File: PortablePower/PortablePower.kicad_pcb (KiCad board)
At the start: 2 copper layers, 44 x 53 mm, 43 parts, among them IC1 SW6208, J1 USB1130-15-A, J2 2137160001, Q1 CSD17313Q2, Q2 CSD17313Q2, Q3 CSD16406Q3, Q4 CSD16406Q3, U1 USBLC6-2SC6, U2 USBLC6-2SC6, U3 BQ297xy

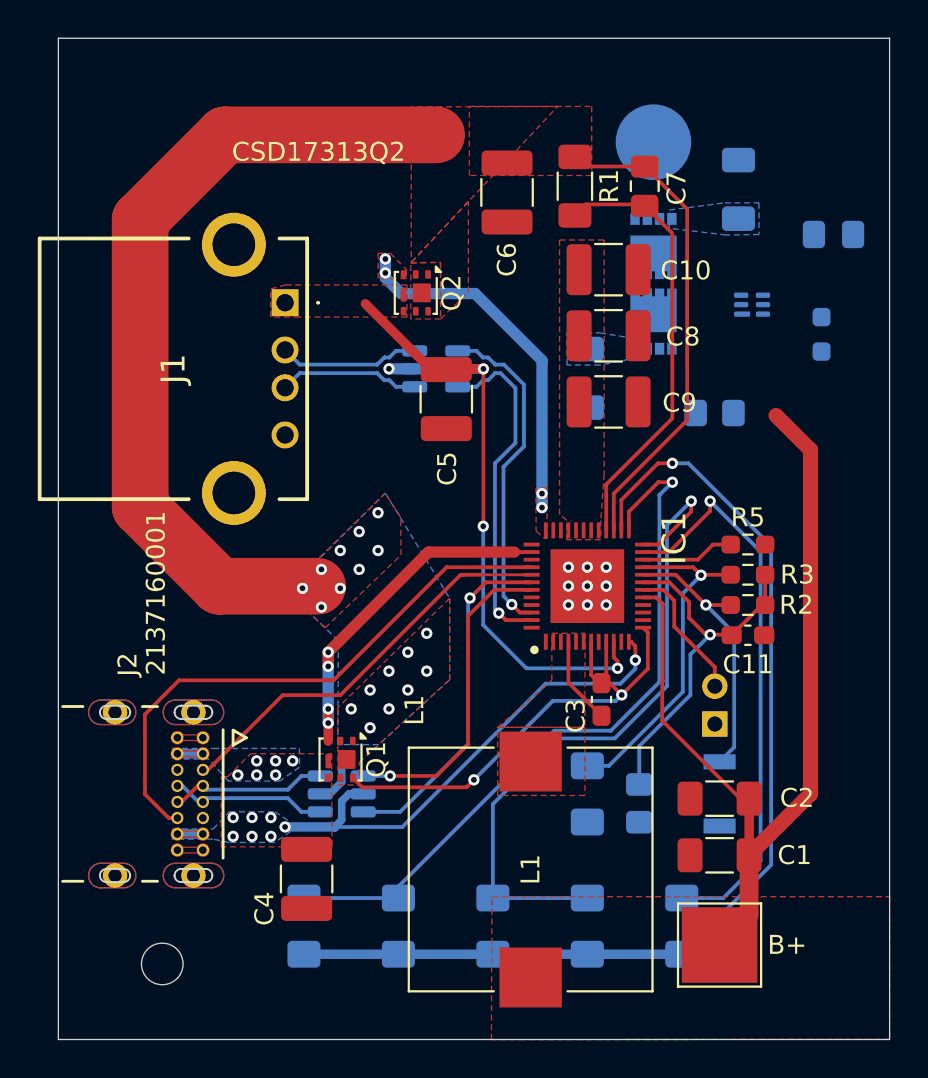
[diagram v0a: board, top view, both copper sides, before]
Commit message: added logo
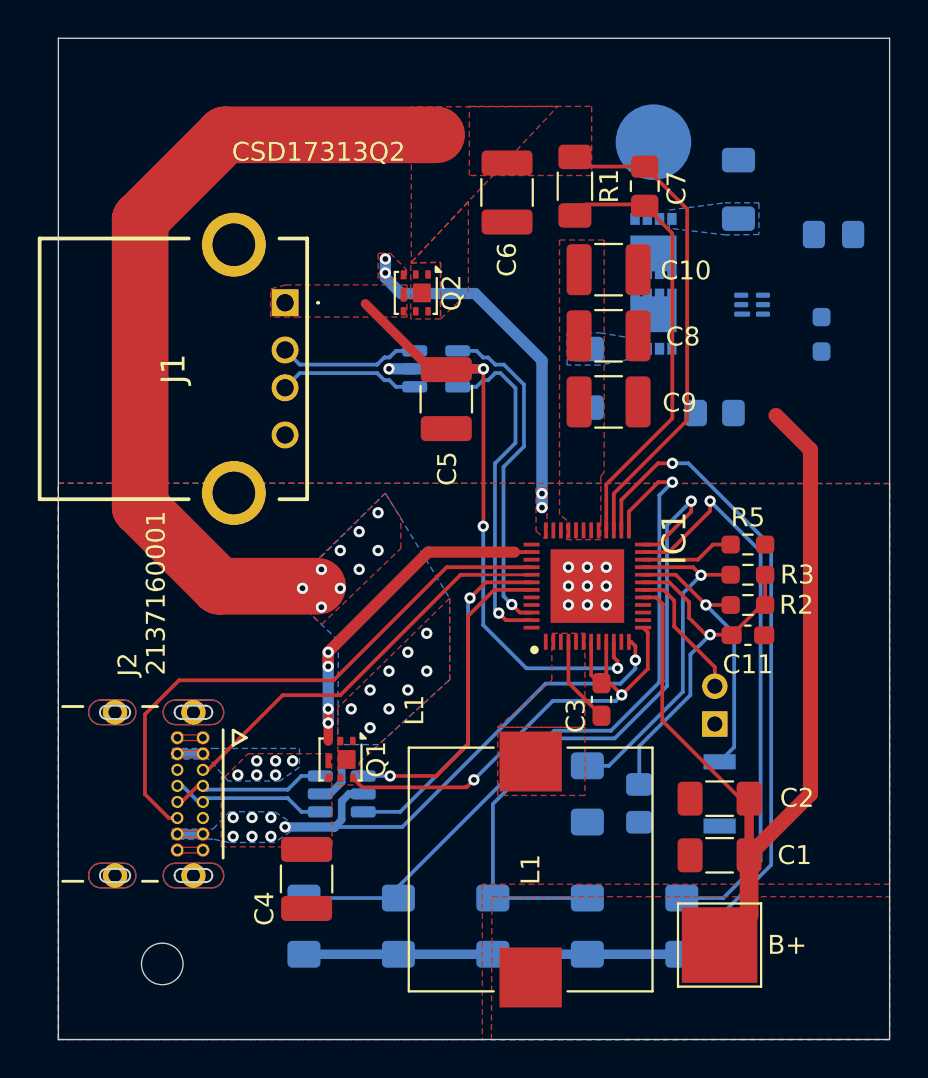
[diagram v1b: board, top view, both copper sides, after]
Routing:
- added copper zone on B.Cu, net GND
- added copper zone on F.Cu, net GND
- added copper zone on B.Cu, net Net-(Q3-G)
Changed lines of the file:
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@@
+	)
+	(segment
+		(start 129.2847 113.5)
+		(end 129.2847 113.4885)
+		(width 0.6)
+		(layer "F.Cu")
+		(net 20)
 	)
 	(segment
@@
 	)
 	(segment
-		(start 129.2847 113.5)
-		(end 134.5847 108.2)
+		(start 129.2847 113.4885)
+		(end 134.5732 108.2)
+		(width 0.6)
+		(layer "F.Cu")
+		(net 20)
+	)
+	(segment
+		(start 134.5732 108.2)
+		(end 139.1412 108.2)
 		(width 0.6)
 		(layer "F.Cu")
@@
 		(end 129.2847 116.5)
 		(width 0.5)
-		(layer "F.Cu")
-		(net 20)
-	)
-	(segment
-		(start 134.5847 108.2)
-		(end 139.1412 108.2)
-		(width 0.6)
 		(layer "F.Cu")
 		(net 20)
@@
 		(name "1")
 		(hatch edge 0.5)
+		(priority 1)
 		(connect_pads yes
 			(clearance 0)
@@
 		(polygon
 			(pts
-				(xy 123.6218 120.101354) (xy 123.952 120.0912) (xy 125.1712 118.872) (xy 129.4638 118.872) (xy 129.489464 123.7996)
-				(xy 123.6218 123.7996)
+				(xy 123.6218 120.101354) (xy 123.820971 120.095229) (xy 125.0442 118.872) (xy 129.4638 118.872)
+				(xy 129.489464 123.7996) (xy 123.6218 123.7996)
 			)
 		)
@@
 		(min_thickness 0.25)
 		(filled_areas_thickness no)
-		(fill
+		(fill yes
 			(thermal_gap 0.5)
 			(thermal_bridge_width 0.5)
@@
 		(name "1")
 		(hatch edge 0.5)
+		(priority 1)
 		(connect_pads yes
 			(clearance 0)
@@
 			(pts
 				(xy 141.9098 107.5436) (xy 141.9098 106.5022) (xy 141.52873 106.218067) (xy 141.52873 91.679346)
-				(xy 143.890941 91.679346) (xy 143.891002 104.0638) (xy 143.7132 106.5276) (xy 143.7132 107.5436)
+				(xy 143.890941 91.679346) (xy 143.891002 103.9876) (xy 143.7132 104.1908) (xy 143.7132 106.5276)
+				(xy 143.7132 107.5436)
 			)
 		)
@@
 	)
 	(zone
+		(net 2)
+		(net_name "GND")
+		(layer "F.Cu")
+		(name "24")
+		(hatch edge 0.5)
+		(connect_pads yes
+			(clearance 0)
+		)
+		(min_thickness 0.25)
+		(filled_areas_thickness no)
+		(fill yes
+			(thermal_gap 0.5)
+			(thermal_bridge_width 0.5)
+			(island_removal_mode 2)
+			(island_area_min 10)
+		)
+		(polygon
+			(pts
+				(xy 114.9858 104.5464) (xy 159.004 104.5718) (xy 159.004 125.7808) (xy 137.4394 125.7808) (xy 137.4394 134.0104)
+				(xy 115.0112 134.0104)
+			)
+		)
+	)
+	(zone
 		(net 22)
 		(net_name "/PD_Control/GATEA1")
@@
 		(polygon
 			(pts
-				(xy 128.1684 111.3028) (xy 129.117893 112.211299) (xy 133.13505 108.3564) (xy 133.1214 106.3752)
+				(xy 128.1684 111.3028) (xy 128.930717 112.032205) (xy 133.132595 108.000046) (xy 133.1214 106.3752)
 				(xy 132.3086 105.0798) (xy 127.21685 110.049492)
 			)
@@
 	)
 	(zone
+		(net 2)
+		(net_name "GND")
+		(layer "B.Cu")
+		(name "1")
+		(hatch edge 0.5)
+		(connect_pads yes
+			(clearance 0)
+		)
+		(min_thickness 0.25)
+		(filled_areas_thickness no)
+		(fill yes
+			(thermal_gap 0.5)
+			(thermal_bridge_width 0.5)
+			(island_removal_mode 2)
+			(island_area_min 10)
+		)
+		(polygon
+			(pts
+				(xy 159.004 104.5718) (xy 159.004 134.0104) (xy 114.9858 134.0104) (xy 114.9858 104.5464)
+			)
+		)
+	)
+	(zone
+		(net 42)
+		(net_name "Net-(Q3-G)")
+		(layer "B.Cu")
+		(name "45")
+		(hatch edge 0.5)
+		(connect_pads yes
+			(clearance 0)
+		)
+		(min_thickness 0.25)
+		(filled_areas_thickness no)
+		(fill yes
+			(thermal_gap 0.5)
+			(thermal_bridge_width 0.5)
+		)
+		(polygon
+			(pts
+				(xy 145.706784 96.929083) (xy 145.706784 97.894283) (xy 143.6784 98.298) (xy 141.9258 98.298) (xy 141.922184 96.598883)
+				(xy 143.6784 96.5962)
+			)
+		)
+	)
+	(zone
+		(net 5)
+		(net_name "/PD_Control/VBUSC")
+		(layer "B.Cu")
+		(name "1")
+		(hatch edge 0.5)
+		(priority 2)
+		(connect_pads yes
+			(clearance 0)
+		)
+		(min_thickness 0.025)
+		(filled_areas_thickness no)
+		(fill yes
+			(thermal_gap 0.5)
+			(thermal_bridge_width 0.5)
+		)
+		(polygon
+			(pts
+				(xy 121.031 119.1514) (xy 121.031 118.5926) (xy 123.19 118.5926) (xy 127.762 118.5926) (xy 127.762 119.5832)
+				(xy 126.7206 120.3198) (xy 123.987338 120.3198) (xy 122.971338 119.1514)
+			)
+		)
+	)
+	(zone
 		(net 43)
 		(net_name "Net-(Q4-G)")
@@
 		(min_thickness 0.25)
 		(filled_areas_thickness no)
-		(fill
-			(thermal_gap 0.5)
-			(thermal_bridge_width 0.5)
-		)
-		(polygon
-			(pts
-				(xy 145.706784 96.929083) (xy 145.706784 97.894283) (xy 143.6784 98.298) (xy 141.9258 98.298) (xy 141.922184 96.598883)
-				(xy 143.6784 96.5962)
-			)
-		)
-	)
-	(zone
-		(net 5)
-		(net_name "/PD_Control/VBUSC")
-		(layer "B.Cu")
-		(name "1")
-		(hatch edge 0.5)
-		(priority 2)
-		(connect_pads yes
-			(clearance 0)
-		)
-		(min_thickness 0.025)
-		(filled_areas_thickness no)
-		(fill yes
-			(thermal_gap 0.5)
-			(thermal_bridge_width 0.5)
-		)
-		(polygon
-			(pts
-				(xy 121.031 119.1514) (xy 121.031 118.5926) (xy 123.19 118.5926) (xy 127.762 118.5926) (xy 127.762 119.5832)
-				(xy 126.7206 120.3198) (xy 123.987338 120.3198) (xy 122.971338 119.1514)
-			)
-		)
-	)
-	(zone
-		(net 43)
-		(net_name "Net-(Q4-G)")
-		(layer "B.Cu")
-		(hatch edge 0.5)
-		(priority 12)
-		(connect_pads yes
-			(clearance 0)
-		)
-		(min_thickness 0.25)
-		(filled_areas_thickness no)
-		(fill
-			(thermal_gap 0.5)
-			(thermal_bridge_width 0.5)
+		(fill yes
+			(thermal_gap 0.5)
+			(thermal_bridge_width 0.5)
